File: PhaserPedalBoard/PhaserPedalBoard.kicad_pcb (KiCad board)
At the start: 4 copper layers, 114 parts, among them J1 Footswitch, J2 SWD Header, J5 In, J6 Out, J7 PowerJack, Q1 BC847, Q2 2N7002, Q4 BC847, Q5 BC857, Q6 BC857, SW1 COLOR, SW2 RST, U1 LMR62014XMF, U2 LM13700, U3 LM13700, U4 AMS1117, U5 TL074, U6 STM32L052K6T6, U7 LM2904

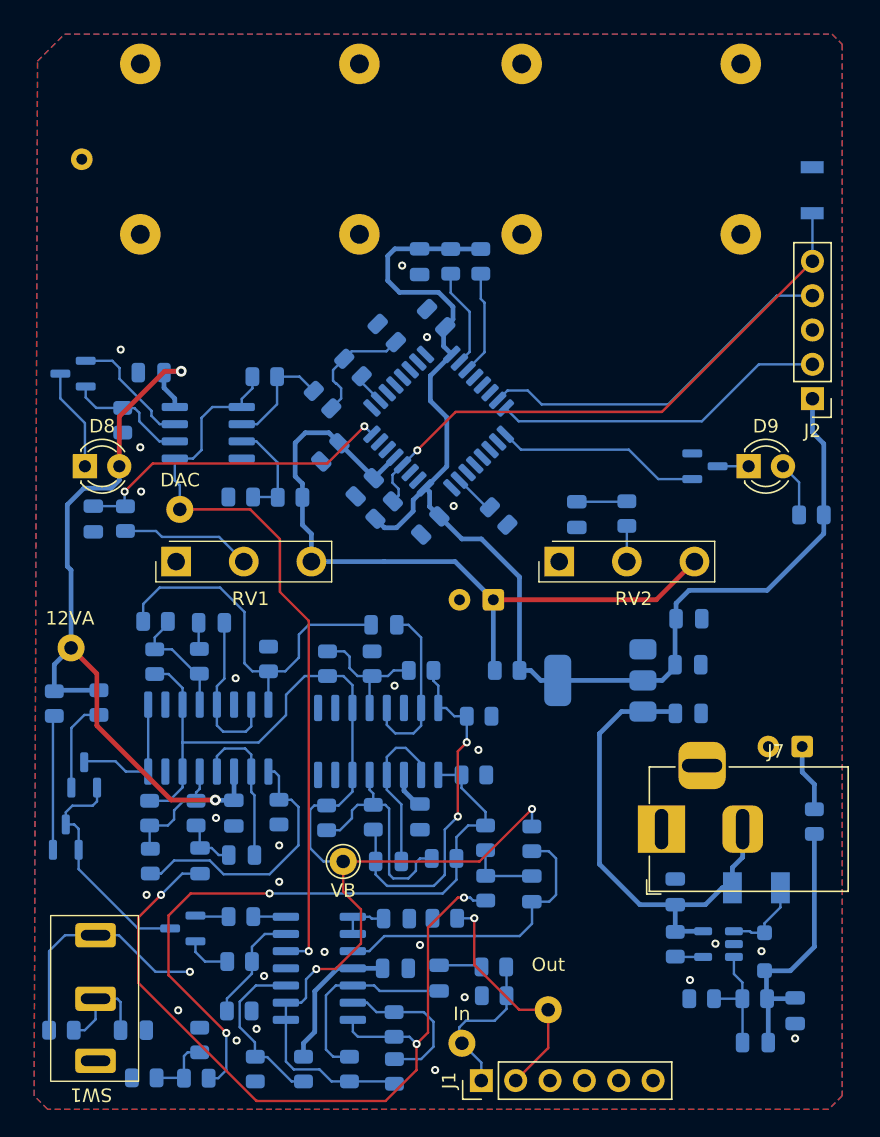
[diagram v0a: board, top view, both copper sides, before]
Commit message: routed, DRC passing
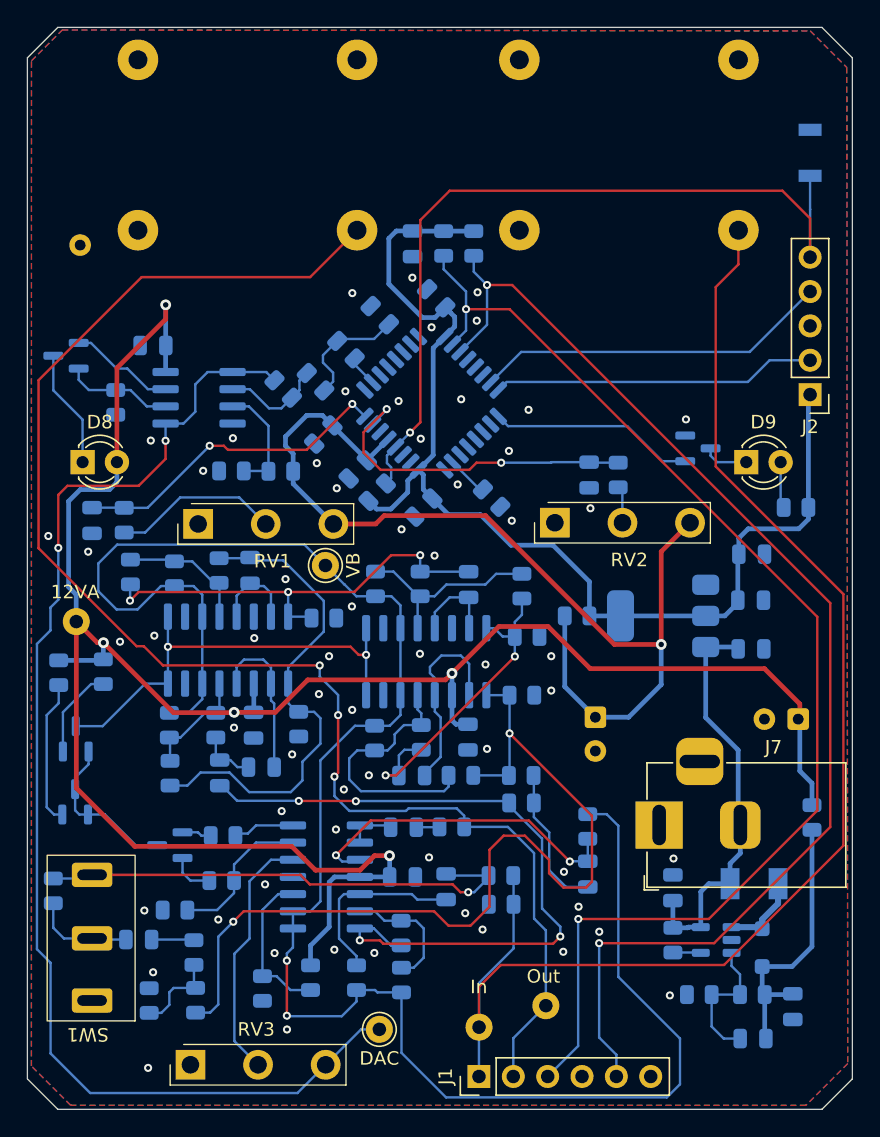
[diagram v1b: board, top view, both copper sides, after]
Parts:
- removed TP5: DAC, TestPoint:TestPoint_THTPad_D2.0mm_Drill1.0mm_VAL
- added RV3: 10kB, Potentiometer_THT:Potentiometer_Alpha_RV16AF_42_Single_Long, F.Cu at (74.1, 113.7)
- added TP3: DAC, TestPoint:TestPoint_THTPad_D2.0mm_Drill1.0mm_VAL, F.Cu at (88.0, 111.1)
- moved TP7 21.9 mm to (84.0, 76.8), turned to -90 degrees
- moved C1 11.5 mm to (104.0, 88.0), turned to -90 degrees
- moved R7 10.3 mm to (63.9, 100.8), turned to 90 degrees
- moved R30 9.97 mm to (74.3, 105.4), turned to -90 degrees
- moved R22 9.71 mm to (98.6, 78.3), turned to 90 degrees
- moved R38 8.84 mm to (72.9, 102.3), turned to 0 degrees
- moved C6 6.93 mm to (94.6, 78.2), turned to -90 degrees
- moved R20 6.88 mm to (91.0, 78.2)
- moved R21 6.88 mm to (87.7, 78.2)
- moved R23 6.88 mm to (99.0, 82.0)
- moved R24 6.88 mm to (91.1, 89.5)
- moved R25 6.88 mm to (87.7, 89.6)
- moved R27 6.88 mm to (98.6, 86.4)
- moved U3 6.88 mm to (91.5, 83.9)
- moved C14 6.88 mm to (94.6, 89.5)
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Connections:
- U5 pad 12: DAC_OUT -> Net-(U5D-+)
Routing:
- net FX_OUT: track 17.8 -> 110.3 mm, vias 1 -> 3
- net +12VA: track 77.0 -> 166.4 mm, vias 2 -> 5
- net FX_IN: track 11.5 -> 100.3 mm
- net BYP_IN: track 7.43 -> 90.9 mm, vias 0 -> 2
- net TAP_IN: track 7.75 -> 91.0 mm, vias 0 -> 2
- net /Analog/VB: track 90.4 -> 143.0 mm
- net DAC_OUT: track 55.8 -> 92.6 mm, vias 1 -> 2
- net /Analog/A: track 10.0 -> 32.9 mm, vias 0 -> 2
- net /Digital/ShapeADC: track 3.72 -> 25.1 mm, vias 0 -> 2
- net +3.3VA: track 54.9 -> 73.8 mm, vias 0 -> 1
- net Net-(U5D-+): track 0.00 -> 18.6 mm
- net /Analog/Stg4: track 49.0 -> 67.2 mm
- net NRST: track 43.5 -> 60.2 mm
- net Net-(SW1-C): track 21.1 -> 36.6 mm
- net /Analog/Stg1: track 21.8 -> 36.9 mm
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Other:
- board outline added: 61 x 80 mm
